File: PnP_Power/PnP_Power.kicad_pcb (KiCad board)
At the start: 2 copper layers, 60 parts, among them J1 Barrel Jack 5mm x 2.5mm 54-00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, U7 VNH5019A-E, U8 LMS78_05-2.0R, U9 SN74LVC2G04DBVR

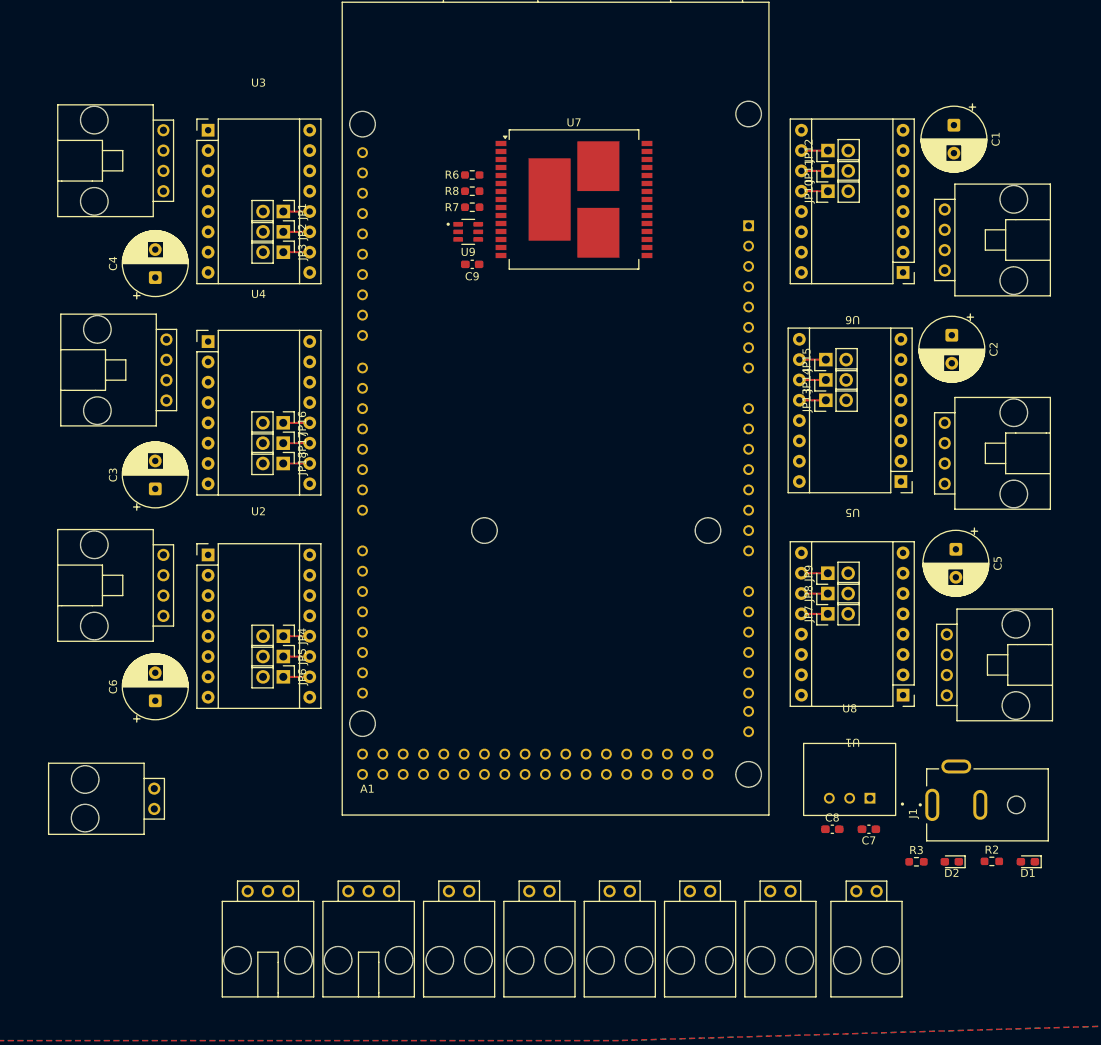
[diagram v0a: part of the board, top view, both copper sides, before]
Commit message: Idek
layouts and stuff and 3d model
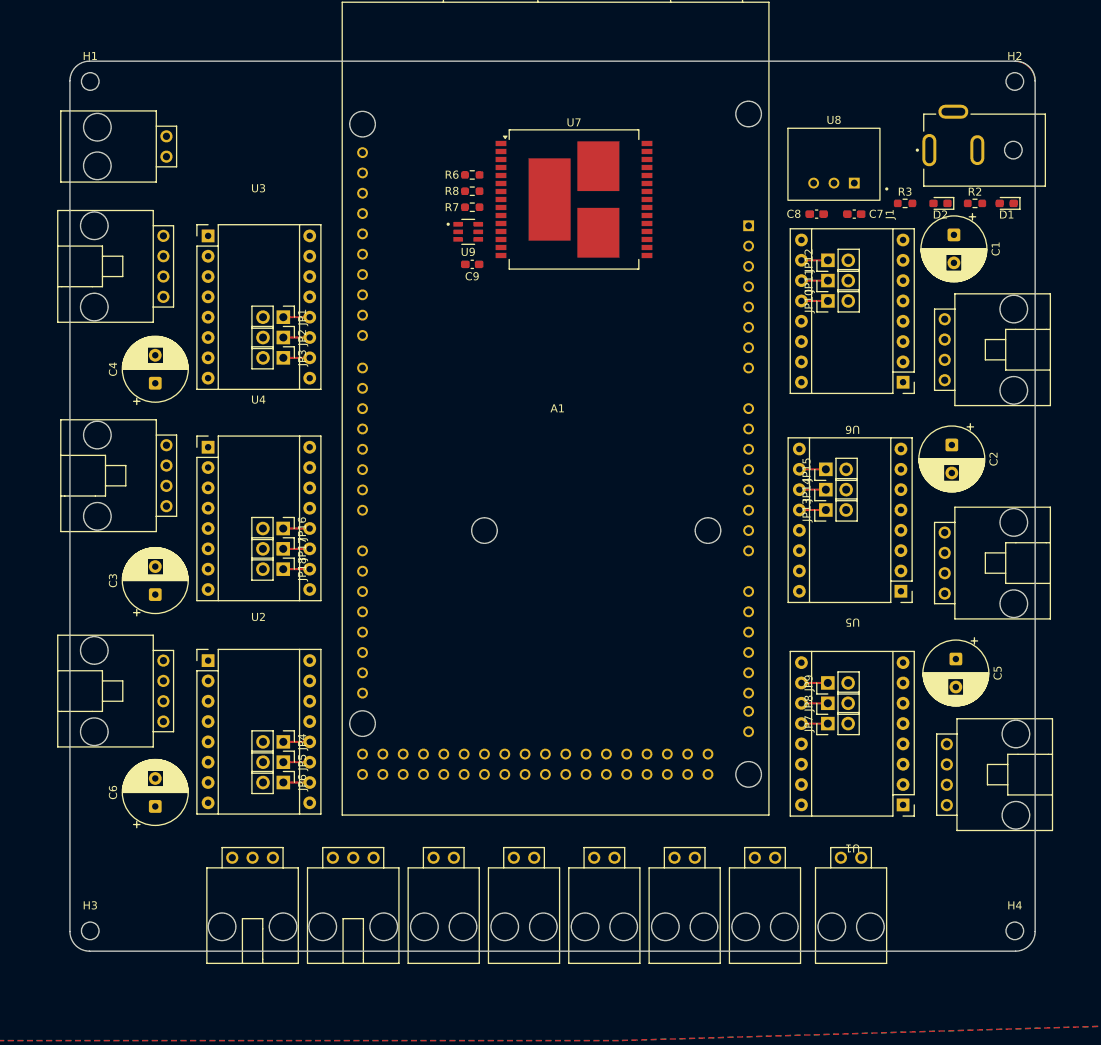
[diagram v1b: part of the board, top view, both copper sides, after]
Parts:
- added H1: MountingHole, MountingHole:MountingHole_2.2mm_M2, F.Cu at (107.7, 52.3)
- added H2: MountingHole, MountingHole:MountingHole_2.2mm_M2, F.Cu at (223.3, 52.3)
- added H3: MountingHole, MountingHole:MountingHole_2.2mm_M2, F.Cu at (107.7, 158.5)
- added H4: MountingHole, MountingHole:MountingHole_2.2mm_M2, F.Cu at (223.3, 158.5)
- moved D1 82.3 mm to (222.2, 67.6)
- moved D2 82.3 mm to (214.0, 67.6)
- moved R3 82.3 mm to (209.6, 67.6)
- moved R2 82.3 mm to (218.3, 67.6)
- moved J1 81.8 mm to (218.6, 60.9)
- moved Conn1 81.5 mm to (117.2, 61.7)
- moved C8 76.9 mm to (198.5, 68.9)
- moved U8 76.9 mm to (200.7, 54.3)
- moved C7 76.9 mm to (203.2, 68.9)
- moved C2 13.7 mm to (215.4, 97.8)
- moved C5 13.7 mm to (215.9, 124.5)
- moved Conn4 13.7 mm to (214.8, 135.2)
- moved Conn6 13.7 mm to (214.5, 108.7)
- moved Conn7 13.7 mm to (214.5, 82.0)
- moved JP13 13.7 mm to (199.6, 105.9)
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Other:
- board outline added: 120.7 x 111.3 mm
